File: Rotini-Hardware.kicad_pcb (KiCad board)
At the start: 4 copper layers, 62 x 21.6 mm, 116 parts, among them J1 Conn_01x02, J2 Conn_01x02, J200 SH_PPM, J201 SH_LED, J202 SH_LED, J60 Conn_Coaxial, Q20 AO3401A, Q30 LBSS84LT1G, Q31 2N7002, Q32 LBSS84LT1G, Q33 2N7002, Q50 SS8050, Q51 SS8050, U1 ESP32-S2, U2 Crystal_ESP32, U20 SY8201CABC, U30 SparkFunH3LIS331DL, U31 H3LIS331DL, U50 CP2102-GMR, U51 USB_C_Receptacle, U52 USB_C_Receptacle, U60 ESP8285H16, U61 Crystal_ESP8285, U70 SX1280, U71 Crystal_SX1280

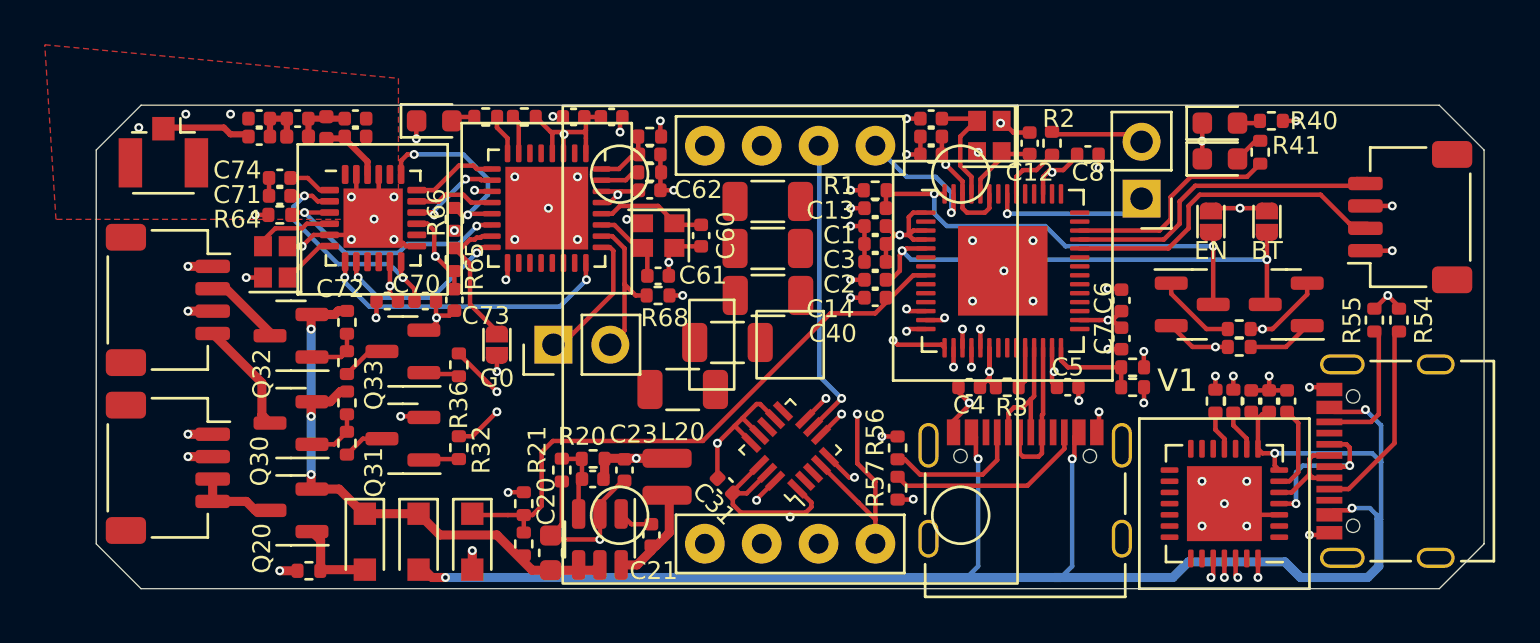
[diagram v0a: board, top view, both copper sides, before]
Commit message: Hardware bought of Rotini V2
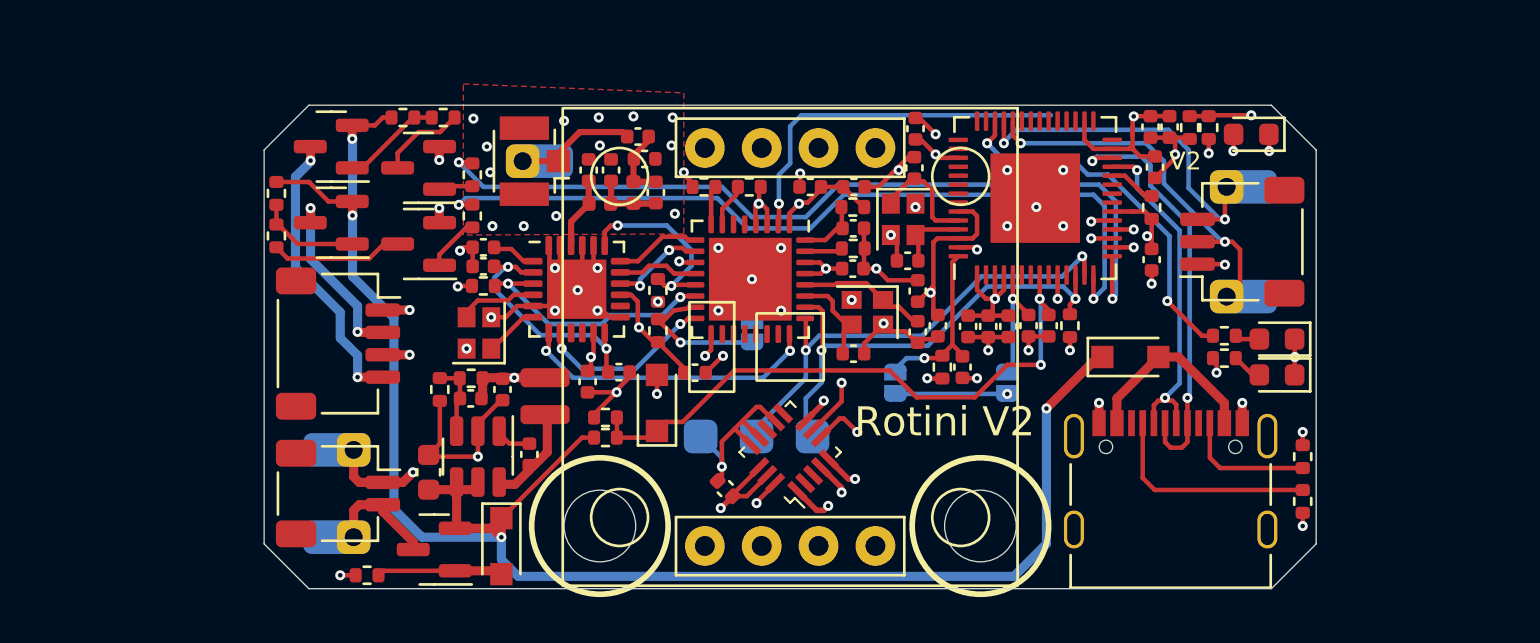
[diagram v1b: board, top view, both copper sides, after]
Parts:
- removed C50, C51: 100nF, Capacitor_SMD:C_0402_1005Metric
- removed C52: 10uF, Capacitor_SMD:C_0402_1005Metric
- removed J1, J2: Conn_01x02, Connector_PinHeader_2.54mm:PinHeader_1x02_P2.54mm_Vertical
- removed J200: SH_PPM, Connector_JST:JST_SH_SM04B-SRSS-TB_1x04-1MP_P1.00mm_Horizontal
- removed Q50, Q51: SS8050, Package_TO_SOT_SMD:SOT-23
- removed R10, R6, R7, R8, R9: 300R, Resistor_SMD:R_1206_3216Metric
- removed R2: 500R, Resistor_SMD:R_0402_1005Metric
- removed R50, R51, R52, R53: 1K, Resistor_SMD:R_0402_1005Metric
- removed R54, R55: 5.1K, Resistor_SMD:R_0402_1005Metric
- removed U50: CP2102-GMR, Package_DFN_QFN:QFN-28-1EP_5x5mm_P0.5mm_EP3.35x3.35mm
- removed U51: USB_C_Receptacle, AlfredoFootprints:USB_TYPE-C-31-M-12
- added ?: , , F.Cu at (8.50, 8.00)
- added ?: , , F.Cu at (-8.50, 8.00)
- added J203: SH_PPM, Connector_JST:JST_SH_SM03B-SRSS-TB_1x03-1MP_P1.00mm_Horizontal, F.Cu at (20.2, -4.70)
- added J205: VIN, AlfredoFootprints:TGD-antenna-THT, B.Cu at (-20.2, 8.50)
- added J206: GND, AlfredoFootprints:TGD-antenna-THT, B.Cu at (-20.2, 4.60)
- added J207: FOO, AlfredoFootprints:TGD-antenna-THT, B.Cu at (20.2, -2.25)
- added J208: BAR, AlfredoFootprints:TGD-antenna-THT, B.Cu at (20.2, -7.15)
- added J61: Conn_01x01_Female, AlfredoFootprints:TGD-antenna-THT, B.Cu at (-11.2, -8.30)
- added TP1: ELRS_TX, AlfredoFootprints:PogoPad1, B.Cu at (1.00, 4.00)
- added TP2: ELRS_RX, AlfredoFootprints:PogoPad1, B.Cu at (-1.50, 4.00)
- added TP3: ELRS_TX, AlfredoFootprints:PogoPad1, B.Cu at (-4.00, 4.00)
- J202: value SH_LED -> SH_POW; footprint Connector_JST:JST_SH_SM04B-SRSS-TB_1x04-1MP_P1.00mm_Horizontal -> Connector_JST:JST_SH_SM02B-SRSS-TB_1x02-1MP_P1.00mm_Horizontal
- JP1, JP2, JP60: moved to B.Cu
- R4: value 7K -> 3.3K
- R60: value 1K -> 12K
- moved D60 36.5 mm to (20.6, -9.50), turned to 180 degrees
- moved D20 32.9 mm to (15.2, 0.45), turned to 0 degrees
- moved R68 18.4 mm to (12.5, -0.95), turned to -90 degrees
- moved R56 18.3 mm to (22.9, 6.90), turned to 90 degrees
- moved R57 18.2 mm to (22.9, 4.90), turned to -90 degrees
- moved C102 17.3 mm to (-6.50, -8.40), turned to 0 degrees
- moved C103 16.9 mm to (-6.80, -9.40)
- moved J60 16.6 mm to (-11.4, -8.30), turned to 180 degrees
- moved C104 16.3 mm to (-6.00, -6.90), turned to 90 degrees
- moved JP2 15.8 mm to (4.70, 1.60), turned to 90 degrees
- moved L102 15.2 mm to (-7.00, -6.90), turned to 90 degrees
- moved R31 15.2 mm to (-15.5, -10.2), turned to 0 degrees
- moved JP1 13.7 mm to (9.70, 1.60), turned to -90 degrees
- moved R30 13.0 mm to (-17.3, -10.2), turned to 0 degrees
- moved L101 12.7 mm to (-8.50, -6.40), turned to 0 degrees
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- renumbered J201 to J204, R36 to R35
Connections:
- J202 pad 2: GND -> Net-(J202-Pad2)
- Q20 pad 3: Net-(J202-Pad3) -> Net-(J202-Pad2)
- R4 pad 1: Net-(R4-Pad1) -> SNS_VER
- R5 pad 2: Net-(R4-Pad1) -> SNS_VER
- U1 pad 10: unconnected-(U1-Pad10) -> SNS_VER
- U1 pad 28: Net-(R4-Pad1) -> unconnected-(U1-Pad28)
- U1 pad 48: Net-(R2-Pad2) -> unconnected-(U1-Pad48)
- U1 pad 49: E_RXD -> unconnected-(U1-Pad49)
- U60 pad 2: unconnected-(U60-Pad2) -> /ExpressLRS-RX/trace_antenna
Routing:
- net VBUS: track 78.5 -> 8.43 mm, vias 6 -> 0
- net VCC: track 26.3 -> 79.0 mm, vias 3 -> 4
- net Net-(D60-Pad2): track 1.07 -> 29.2 mm, vias 0 -> 2
- net E_RXD: track 27.5 -> 0.00 mm, vias 2 -> 0
- net E_TXD: track 27.4 -> 0.00 mm, vias 1 -> 0
- net SNS_VER: track 0.00 -> 25.8 mm, vias 0 -> 2
- net E_IO0: track 22.6 -> 5.33 mm, vias 2 -> 1
- net CP_RTS: track 16.8 -> 0.00 mm, vias 2 -> 0
- net /ExpressLRS-RX/trace_antenna: track 0.00 -> 16.5 mm, vias 0 -> 1
- net CP_DTR: track 16.3 -> 0.00 mm, vias 2 -> 0
- net LED_1: track 23.7 -> 38.2 mm
- net P_MISO: track 21.8 -> 35.4 mm
- net LED_2: track 22.8 -> 36.4 mm
- net E_EN: track 20.6 -> 7.79 mm, vias 2 -> 1
- net P_MOSI: track 15.5 -> 27.6 mm
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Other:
- board size 62 x 21.6 mm -> 47 x 21.6 mm
- board text added: "3V3"
- board text added: "ANT"
- board text added: "Alfredo Systems © 2022 Rotini V2"
- board text added: "BAR"
- board text added: "CS2"
- board text added: "FOO"
- board text added: "G"
- board text added: "GND"
- board text added: "MISO"
- board text added: "MOSI"
- board text added: "RX"
- board text added: "Rotini V2"
- board text added: "SCK"
- board text added: "TX"
- board text added: "V2"
- board text added: "VIN"
- board text added: "X"
- board text removed: "Rotini V1"
- board text removed: "V1"
- board text removed: "© 2022 Alfredo Systems"
